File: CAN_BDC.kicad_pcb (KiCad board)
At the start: 2 copper layers, 26 x 28 mm, 30 parts, among them P1 CONN_01X02, P2 CONN_01X05, P3 CONN_01X02, P4 CONN_01X02, P5 CONN_01X02, P6 CONN_01X02, P7 CONN_01X04, P8 CONN_01X01, U1 PSD2CAN, U2 SN65HVD232D, U3 POLOLU_A4988, U4 STM32F042G4U6, U5 MC33063

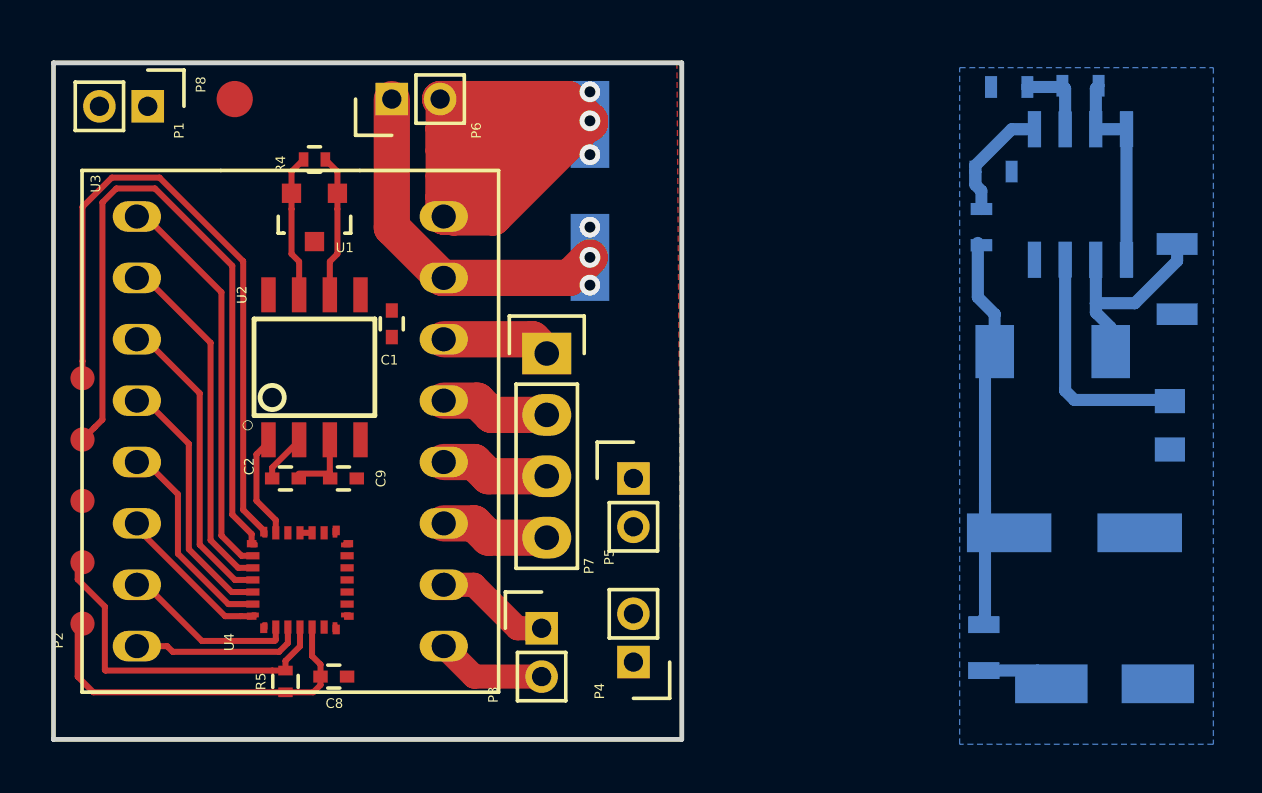
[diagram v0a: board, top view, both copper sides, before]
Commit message: Fids addition
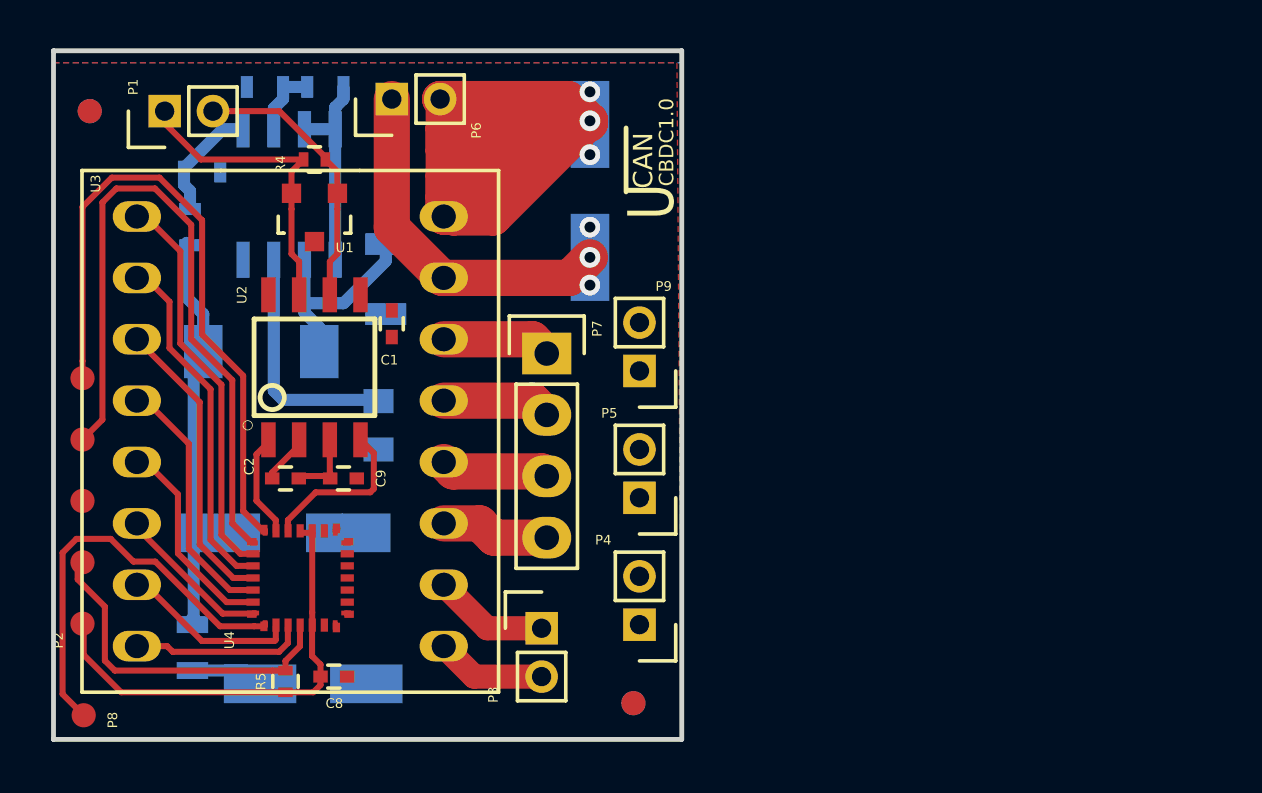
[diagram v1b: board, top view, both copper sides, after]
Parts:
- added P9: CONN_01X02, Pin_Headers:Pin_Header_Straight_1x02_Pitch2.00mm, F.Cu at (161.7, 96.3)
- added f1: fiducial, Fiducials:Fiducial_1mm_Dia_2.54mm_Outer_CopperTop, F.Cu at (161.4, 110.0)
- added f2: fiducial, Fiducials:Fiducial_1mm_Dia_2.54mm_Outer_CopperTop, F.Cu at (138.9, 85.5)
- added f3: fiducial, Fiducials:Fiducial_1mm_Dia_2.54mm_Outer_CopperBottom, F.Cu at (161.4, 110.0)
- added f4: fiducial, Fiducials:Fiducial_1mm_Dia_2.54mm_Outer_CopperBottom, F.Cu at (138.9, 85.5)
- moved C5 32.8 mm to (150.8, 98.5)
- moved C6 32.8 mm to (146.9, 103.0)
- moved C7 32.8 mm to (148.2, 109.2)
- moved D1 32.8 mm to (151.2, 92.5)
- moved L1 32.8 mm to (148.4, 95.5)
- moved L2 32.8 mm to (143.2, 107.8)
- moved R1 32.8 mm to (143.6, 88.0)
- moved R3 32.8 mm to (143.1, 90.3)
- moved U5 32.8 mm to (147.2, 89.0)
- moved R2 31.3 mm to (148.7, 84.5)
- moved R6 30.8 mm to (146.2, 84.5)
- moved P8 26.3 mm to (138.7, 110.5)
- moved P4 1.57 mm to (161.7, 106.8)
- moved P5 0.84 mm to (161.7, 101.5), turned to 180 degrees
- moved P1 0.73 mm to (142.0, 85.5), turned to 90 degrees
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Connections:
- P5 pad 1: Net-(P5-Pad1) -> /GPIO1
- P5 pad 2: Net-(P5-Pad2) -> /GPIO2
- U4 pad 10: Net-(U4-Pad10) -> /GPIO1
- U4 pad 11: Net-(U4-Pad11) -> /GPIO2
- U4 pad 12: Net-(U4-Pad12) -> /GPIO3
- U4 pad 13: Net-(U4-Pad13) -> /GPIO4
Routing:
- net Net-(P8-Pad1): track 0.00 -> 17.2 mm
- net CAN_RX: track 0.31 -> 7.18 mm
- net Net-(P1-Pad1): track 5.54 -> 12.4 mm
- net Net-(P1-Pad2): track 5.54 -> 11.1 mm
- net +3V3: track 27.3 -> 30.7 mm
- net CAN_MOD: track 0.00 -> 0.57 mm
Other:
- board size 26 x 28 mm -> 26 x 28.5 mm
